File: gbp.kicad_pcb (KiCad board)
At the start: 2 copper layers, 63.5 x 119.4 mm, 5 parts

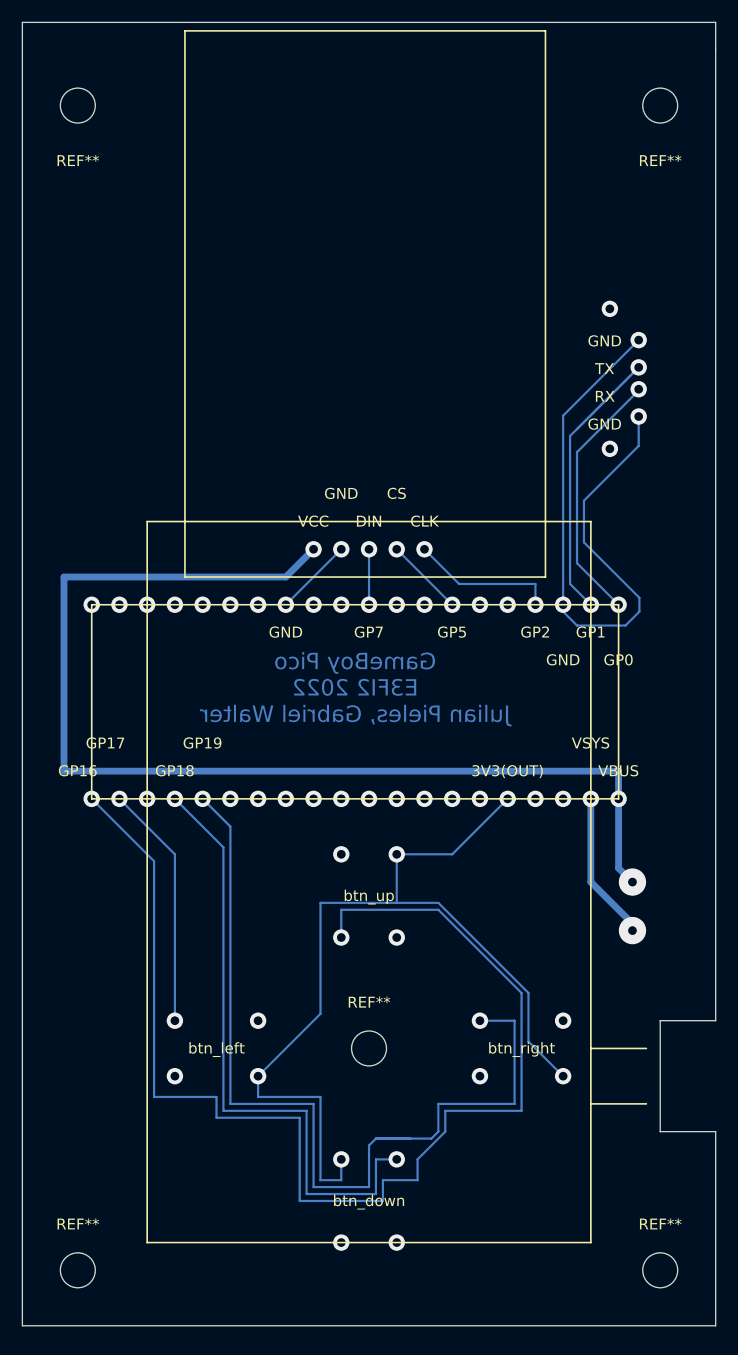
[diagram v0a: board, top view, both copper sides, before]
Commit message: circuitboard update
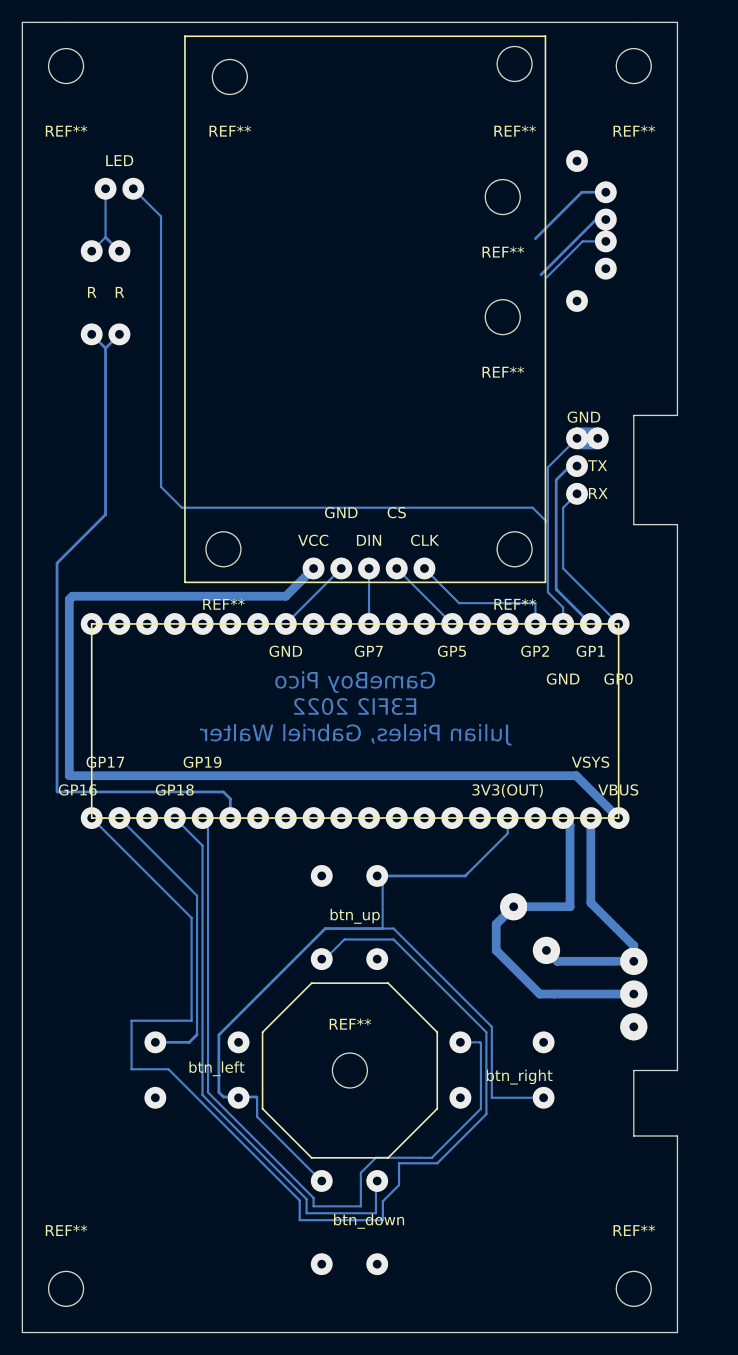
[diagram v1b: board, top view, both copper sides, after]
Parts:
- added REF**: MountingHole_3.2mm_M3, MountingHole:MountingHole_3.2mm_M3, F.Cu at (80.6, 83.8)
- added REF**: MountingHole_3.2mm_M3, MountingHole:MountingHole_3.2mm_M3, F.Cu at (80.6, 39.4)
- added REF**: MountingHole_3.2mm_M3, MountingHole:MountingHole_3.2mm_M3, F.Cu at (54.0, 83.8)
- added REF**: MountingHole_3.2mm_M3, MountingHole:MountingHole_3.2mm_M3, F.Cu at (54.6, 40.6)
- added REF**: MountingHole_3.2mm_M3, MountingHole:MountingHole_3.2mm_M3, F.Cu at (79.6, 51.6)
- added REF**: MountingHole_3.2mm_M3, MountingHole:MountingHole_3.2mm_M3, F.Cu at (79.6, 62.6)
- moved REF** 4.35 mm to (91.6, 39.6)
- moved REF** 3.78 mm to (39.6, 39.6)
- moved REF** 2.96 mm to (91.6, 151.6)
- moved REF** 2.67 mm to (65.6, 131.6)
- moved REF** 2.01 mm to (39.6, 151.6)
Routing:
- net (no net): track 627.8 -> 729.1 mm, vias 69 -> 82
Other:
- board size 63.5 x 119.4 mm -> 60 x 120 mm
- board text added: "LED"
- board text added: "R"
